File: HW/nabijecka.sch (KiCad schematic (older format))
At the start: 9 parts, among them U5 TP4056

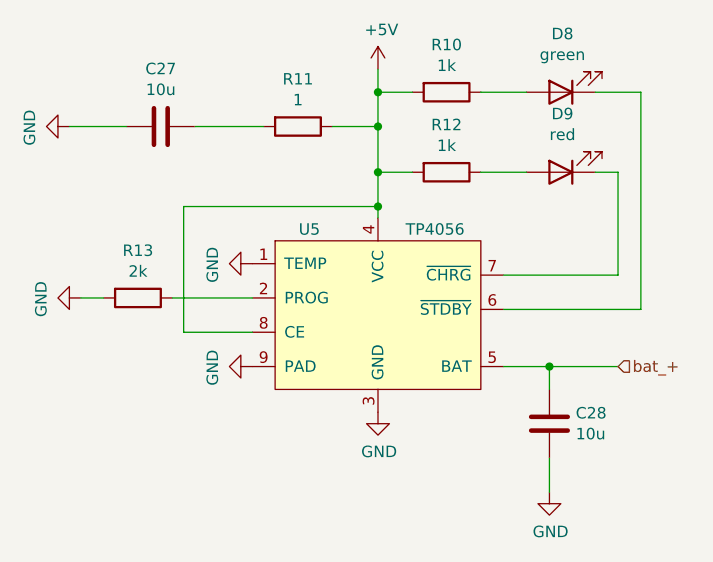
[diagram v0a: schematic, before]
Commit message: change path
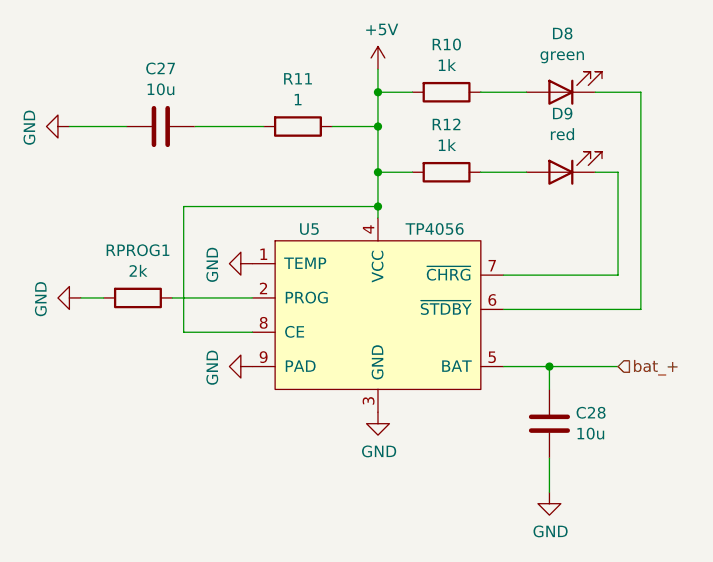
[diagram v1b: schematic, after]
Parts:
- renumbered R13 to RPROG1
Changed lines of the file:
@@
 	4500 2800 4500 2650
 $Comp
-L Device:R R13
+L Device:R RPROG1
 U 1 1 5F721EB5
 P 3450 3200
-F 0 "R13" V 3243 3200 50  0000 C CNN
+F 0 "RPROG1" V 3243 3200 50  0000 C CNN
 F 1 "2k" V 3334 3200 50  0000 C CNN
 F 2 "Resistor_SMD:R_0402_1005Metric" V 3380 3200 50  0001 C CNN

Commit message: repair project
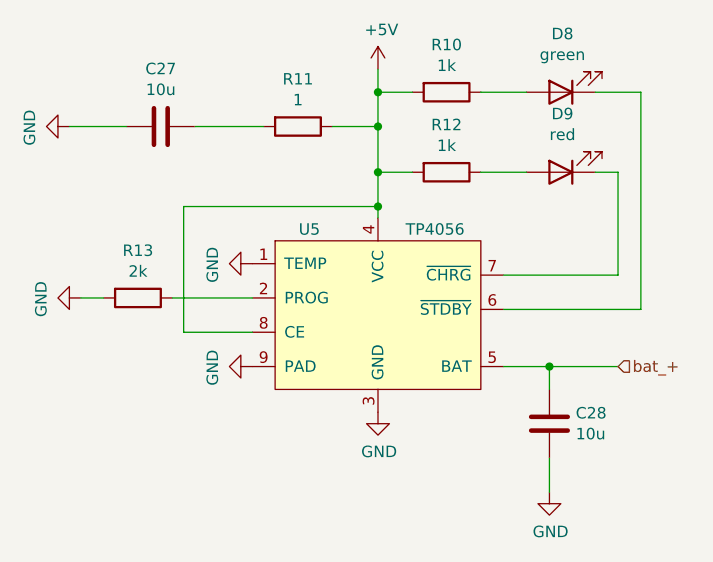
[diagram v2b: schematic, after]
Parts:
- renumbered RPROG1 to R13
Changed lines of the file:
@@
 	4500 2800 4500 2650
 $Comp
-L Device:R RPROG1
+L Device:R R13
 U 1 1 5F721EB5
 P 3450 3200
-F 0 "RPROG1" V 3243 3200 50  0000 C CNN
+F 0 "R13" V 3243 3200 50  0000 C CNN
 F 1 "2k" V 3334 3200 50  0000 C CNN
 F 2 "Resistor_SMD:R_0402_1005Metric" V 3380 3200 50  0001 C CNN
